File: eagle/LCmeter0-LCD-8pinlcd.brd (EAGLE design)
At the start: 58.4 x 48.2 mm, 27 parts, among them IC1 PIC16F876A-X/SP, K2 DS2Y, Q1 20MHz, Q2 BC547CBE, SW1 SPST, X1 FREQ, X2 L/C

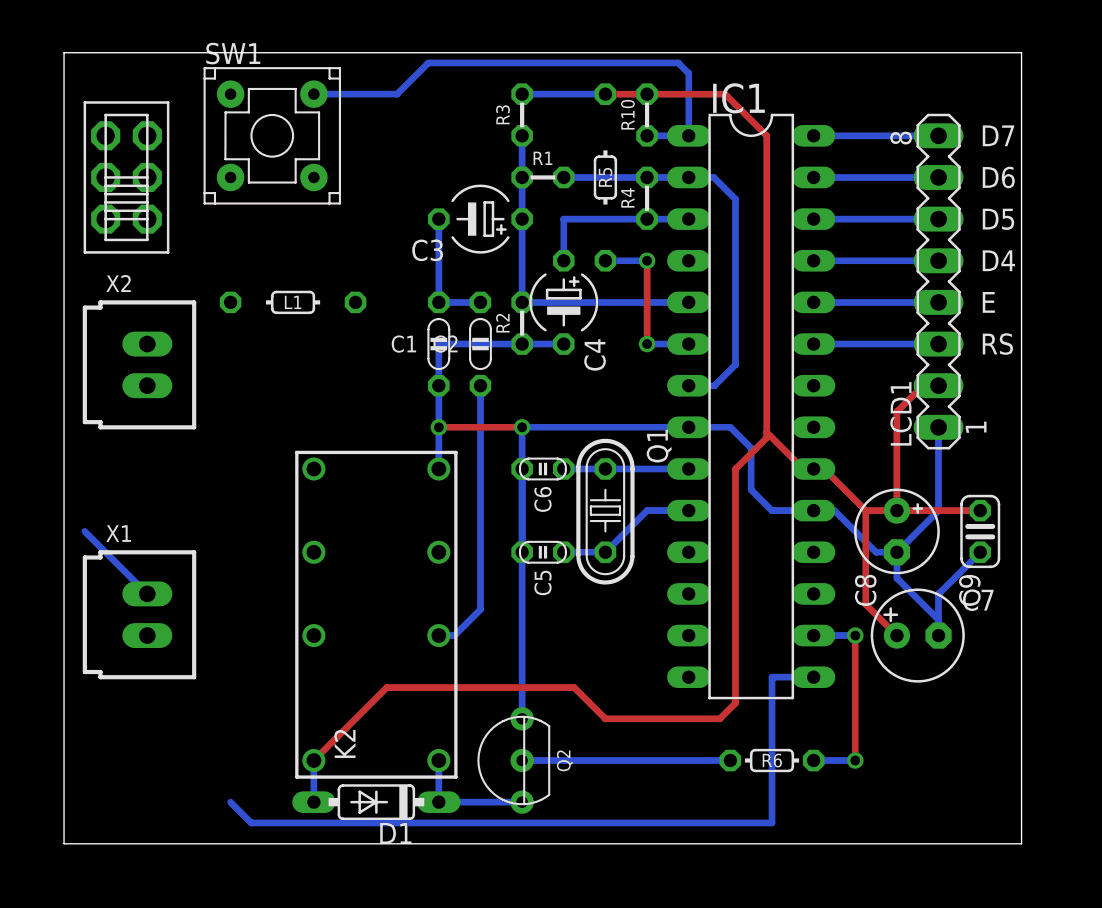
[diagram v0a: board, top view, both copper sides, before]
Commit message: ...
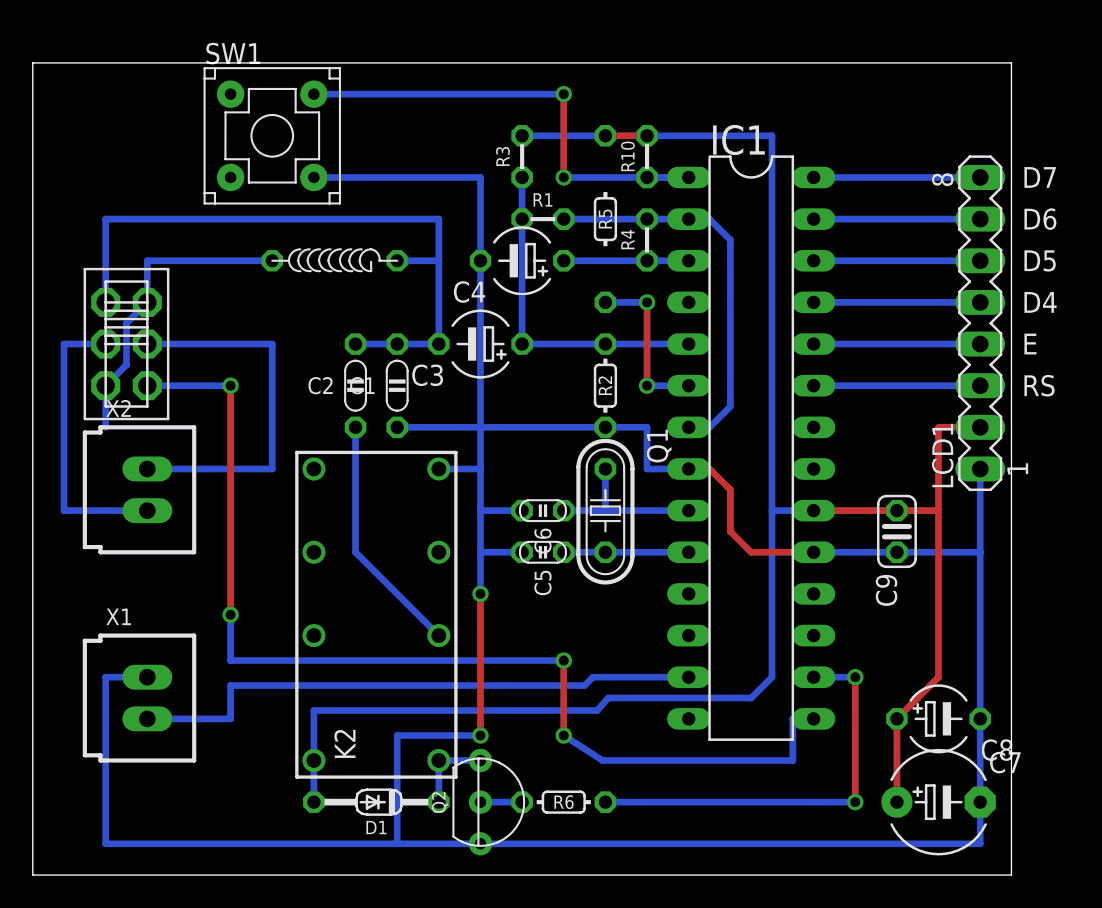
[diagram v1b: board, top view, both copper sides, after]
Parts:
- C7: device rcl:E2,5-6 -> c:E5-6
- C8: device rcl:E2,5-5 -> c:E5-4
- D1: device diode:DO35-7 -> d:DO34-7
- L1: device r:0202/7 -> r:L-02/7
- R2: device r:0202/2V -> r:0202/5
- moved R6 13.0 mm to (30.5, 2.54)
- moved C8 11.7 mm to (53.3, 7.62), turned to 0 degrees
- moved C7 10.2 mm to (53.3, 2.54)
- moved S1 10.2 mm to (3.81, 30.5), turned to 0 degrees
- moved C2 8.03 mm to (17.8, 27.9)
- moved C3 7.62 mm to (25.4, 30.5)
- moved X2 7.62 mm to (5.08, 21.6)
- moved R2 6.35 mm to (33.0, 27.9)
- moved C9 5.08 mm to (50.8, 19.1)
- moved X1 5.08 mm to (5.08, 8.89)
- moved Q2 3.59 mm to (25.4, 2.54), turned to 270 degrees
- moved L1 3.59 mm to (16.5, 35.6), turned to 90 degrees
- moved C1 3.59 mm to (20.3, 27.9)
- moved C4 3.59 mm to (27.9, 35.6), turned to 180 degrees
- moved LCD1 3.59 mm to (55.9, 31.8)
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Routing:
- net GND: track 97.0 -> 194.1 mm
- net FREQ: track 0.00 -> 35.3 mm
- net N$2: track 7.62 -> 40.6 mm
- net M-: track 0.00 -> 22.9 mm
- net /LC: track 45.0 -> 65.0 mm, vias 0 -> 4
- net N$7: track 0.00 -> 18.8 mm
- net M+: track 0.00 -> 17.8 mm
- net RC5: track 12.7 -> 25.4 mm, vias 2 -> 3
- net N$5: track 12.7 -> 2.54 mm
- net /RELAY: track 7.62 -> 5.08 mm
- net RS: track 7.62 -> 10.2 mm
- net OSC1: track 7.62 -> 10.2 mm
- net E: track 7.62 -> 10.2 mm
- net D7: track 7.62 -> 10.2 mm
- net D6: track 8.89 -> 11.4 mm
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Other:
- board size 58.4 x 48.2 mm -> 59.7 x 49.5 mm
